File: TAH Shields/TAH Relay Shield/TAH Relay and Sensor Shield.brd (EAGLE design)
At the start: 86.8 x 54 mm, 40 parts, among them T1 2N3904, T2 2N3904

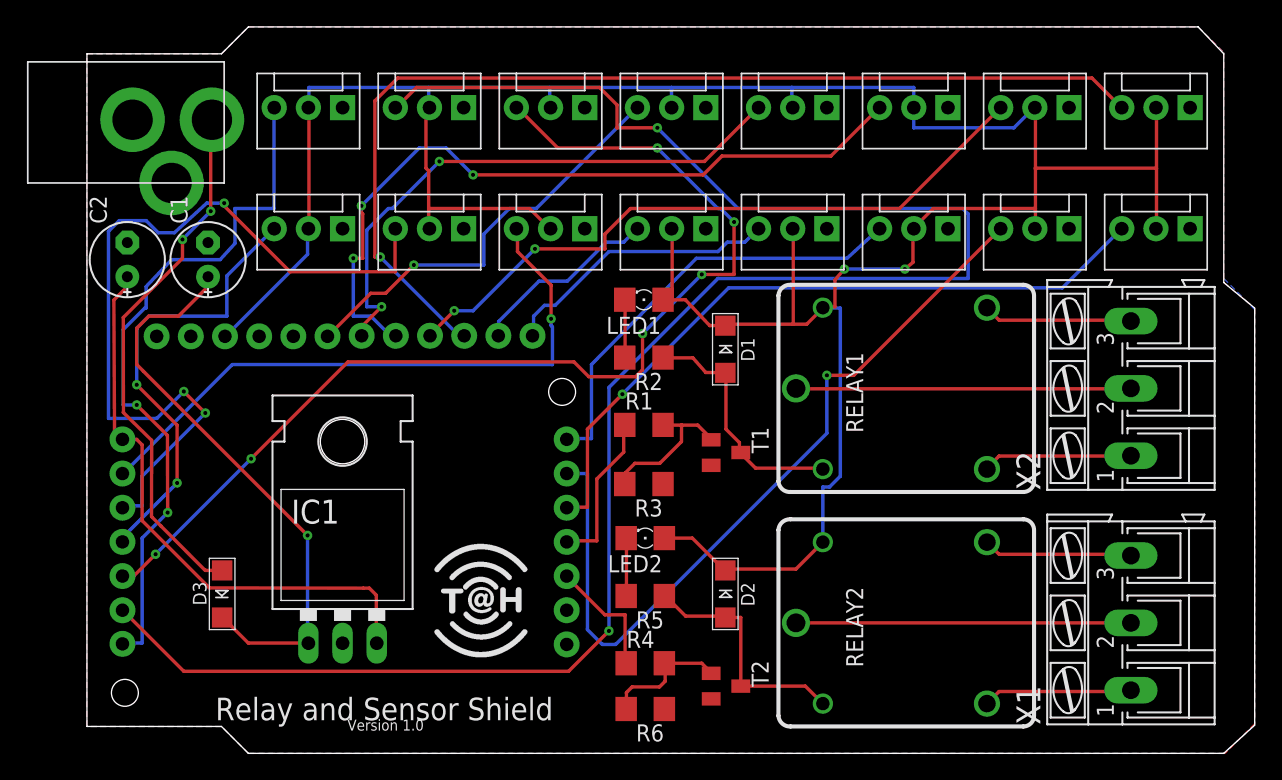
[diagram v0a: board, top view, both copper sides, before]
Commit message: TAH Shields new version update
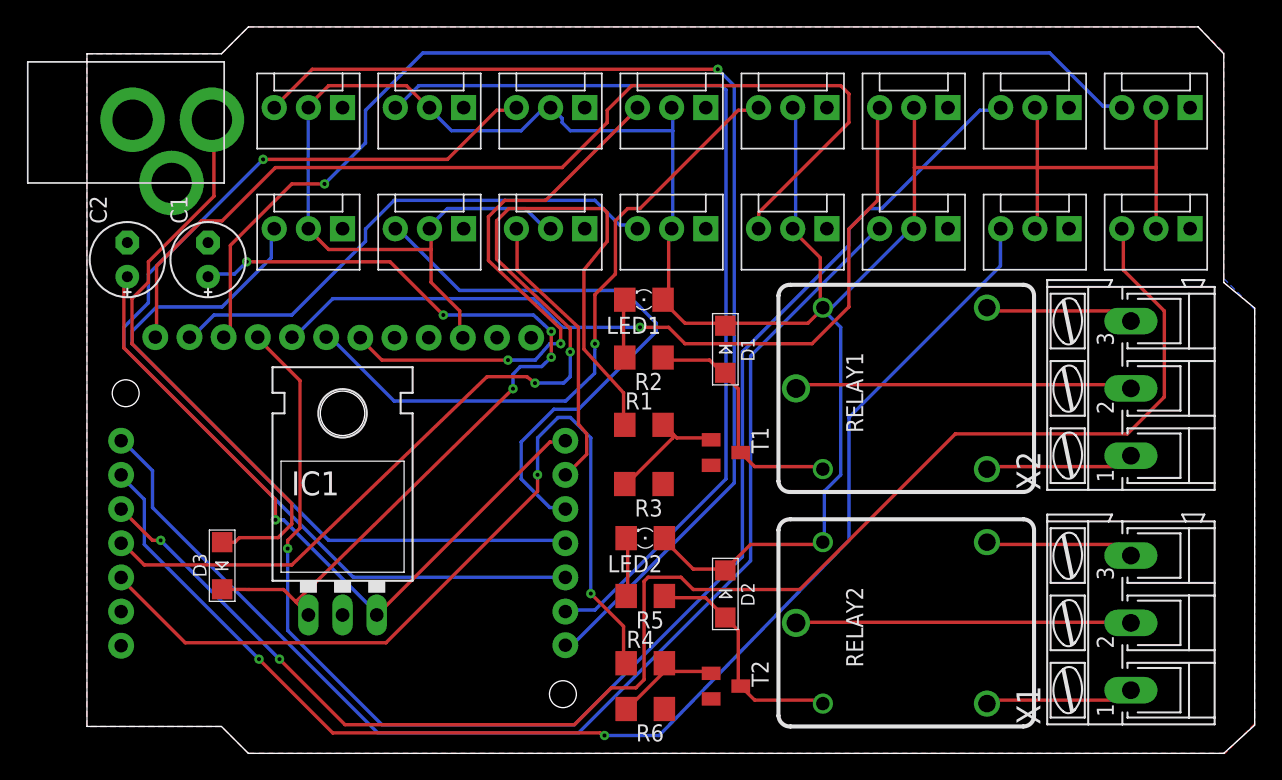
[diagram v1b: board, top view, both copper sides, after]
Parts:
- removed U$4, U$5: (no value), TAH:TAHLOGO
- added U$2: (no value), TAH:TAHLOGO
- moved D3 2.10 mm to (10.0, 14.1)
- moved IC1 2.10 mm to (19.0, 14.1)
- moved U$1 0.14 mm to (19.1, 5.46), flipped to the bottom
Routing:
- net A4: track 140.3 -> 70.3 mm, vias 2 -> 0
- net D3: track 11.8 -> 80.2 mm, vias 0 -> 2
- net D4: track 53.2 -> 113.2 mm, vias 1 -> 2
- net D6: track 32.9 -> 91.4 mm
- net D10: track 50.1 -> 108.1 mm, vias 2 -> 1
- net D2: track 9.23 -> 64.7 mm, vias 0 -> 2
- net D7: track 20.9 -> 75.9 mm
- net D5: track 59.6 -> 98.1 mm, vias 1 -> 2
- net A5: track 52.5 -> 83.0 mm, vias 2 -> 1
- net A0: track 46.6 -> 21.2 mm, vias 1 -> 0
- net D8: track 14.2 -> 39.0 mm
- net N$5: track 43.2 -> 64.3 mm, vias 1 -> 5
- net A2: track 33.8 -> 54.2 mm, vias 2 -> 0
- net A1: track 61.3 -> 43.3 mm, vias 3 -> 0
- net 5V: track 212.4 -> 200.0 mm, vias 2 -> 0
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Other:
- board text added: "http://www.tah.io/start"
- board text removed: "by Revealing Hour Creations"
